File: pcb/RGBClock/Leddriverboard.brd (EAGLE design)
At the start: 68 x 41 mm, 37 parts, among them U1 LP3878MR-ADJ, U2 P82B96DR, U3 PCA9685PW, U4 ZXLD1362ET5TA, U5 ZXLD1362ET5TA, U6 ZXLD1362ET5TA, X1 43045-0400, X2 43045-0600

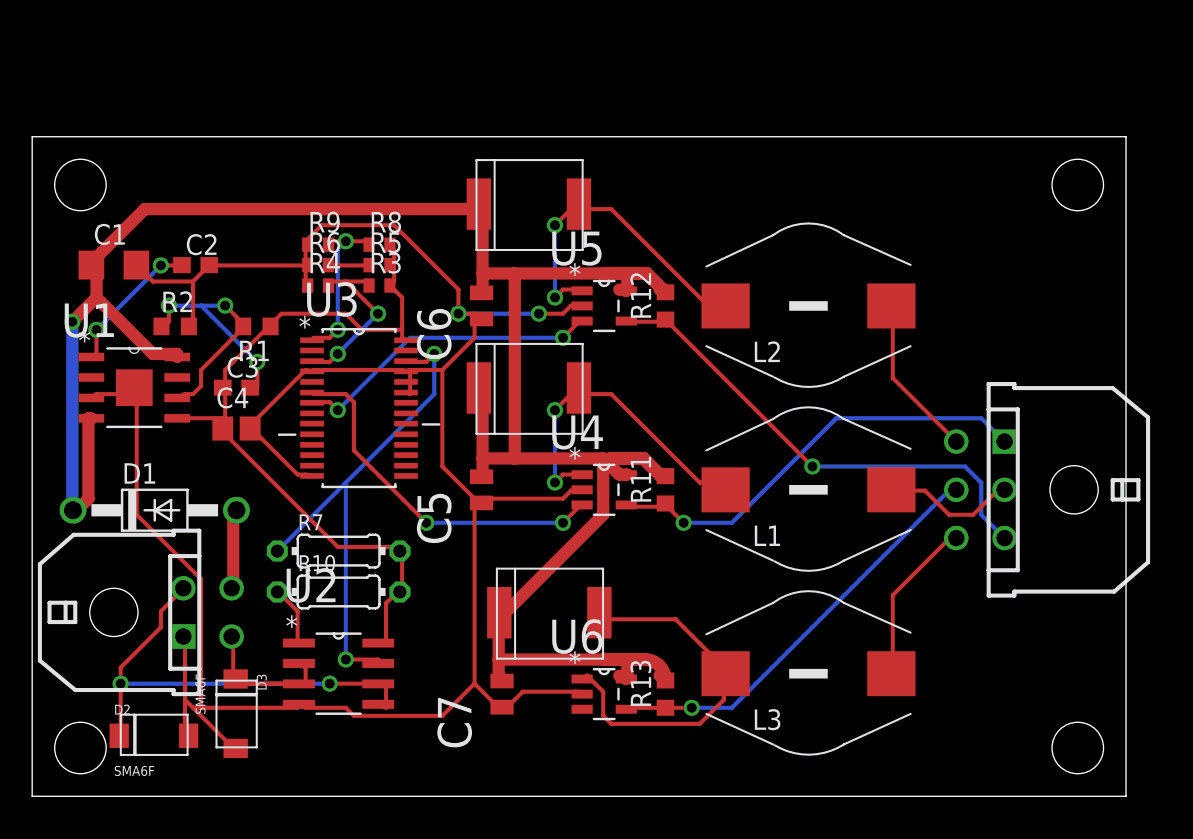
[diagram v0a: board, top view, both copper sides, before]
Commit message: Beta version master pcb (not complete routed !)
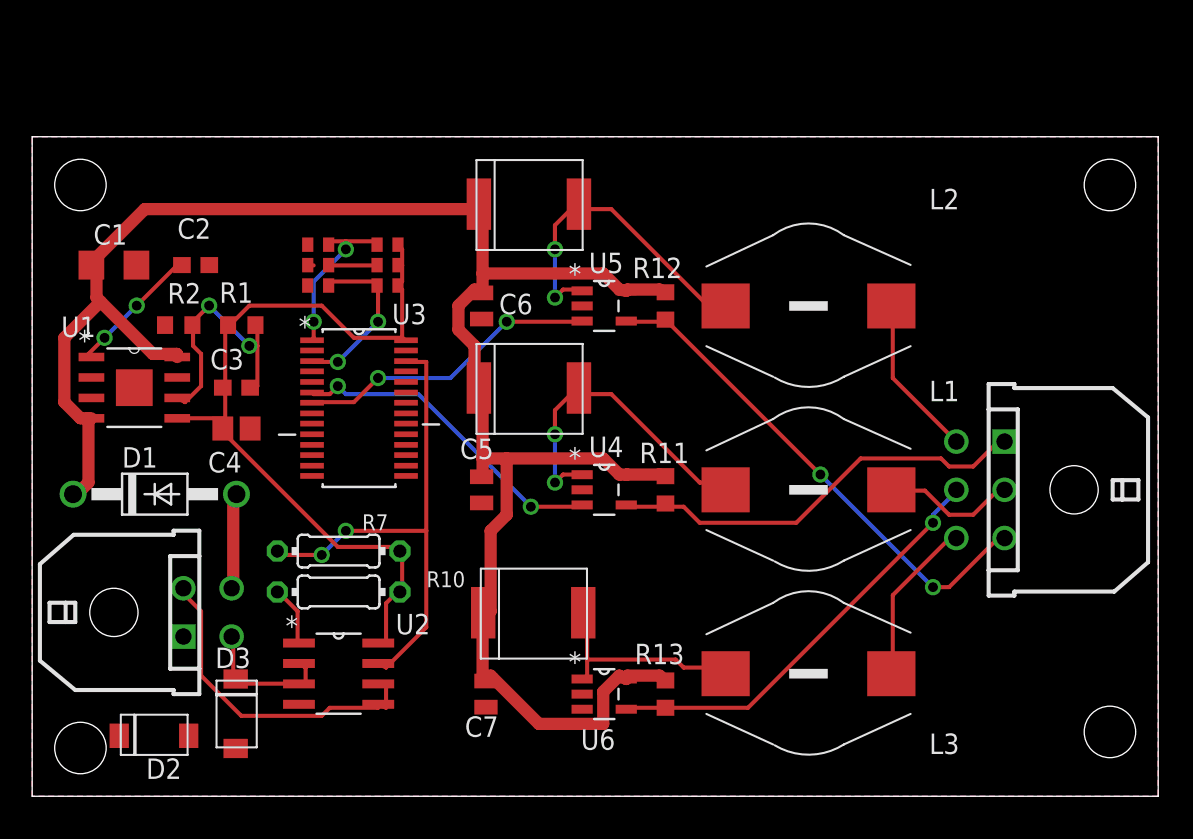
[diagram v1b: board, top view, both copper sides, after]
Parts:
- moved C7 1.00 mm to (28.2, 6.35)
- moved D1 1.00 mm to (7.62, 18.8)
- moved D6 1.00 mm to (29.5, 11.4)
- moved R1 0.94 mm to (13.0, 29.3), turned to 0 degrees
- moved R3 0.50 mm to (22.1, 31.8)
- moved R5 0.50 mm to (22.1, 33.0)
- moved R8 0.50 mm to (22.1, 34.3)
- moved R2 0.23 mm to (9.11, 29.3), turned to 180 degrees
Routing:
- net GND: track 153.7 -> 0.37 mm, vias 2 -> 0
- net VCC: track 135.1 -> 121.6 mm, vias 1 -> 0
- net N$19: track 22.9 -> 13.5 mm
- net N$22: track 29.3 -> 20.8 mm, vias 2 -> 0
- net N$24: track 20.2 -> 15.9 mm, vias 3 -> 2
- net N$8: track 22.3 -> 20.2 mm
- net +5V: track 48.1 -> 50.0 mm
- net N$4: track 30.3 -> 31.7 mm, vias 1 -> 2
- net N$25: track 4.97 -> 5.97 mm
- net N$1: track 27.4 -> 26.6 mm, vias 1 -> 0
- net N$42: track 2.64 -> 3.14 mm
- added copper zone on layer 1, net GND
- added copper zone on layer 16, net GND
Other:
- board size 68 x 41 mm -> 70 x 41 mm

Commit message: Just before freerouter
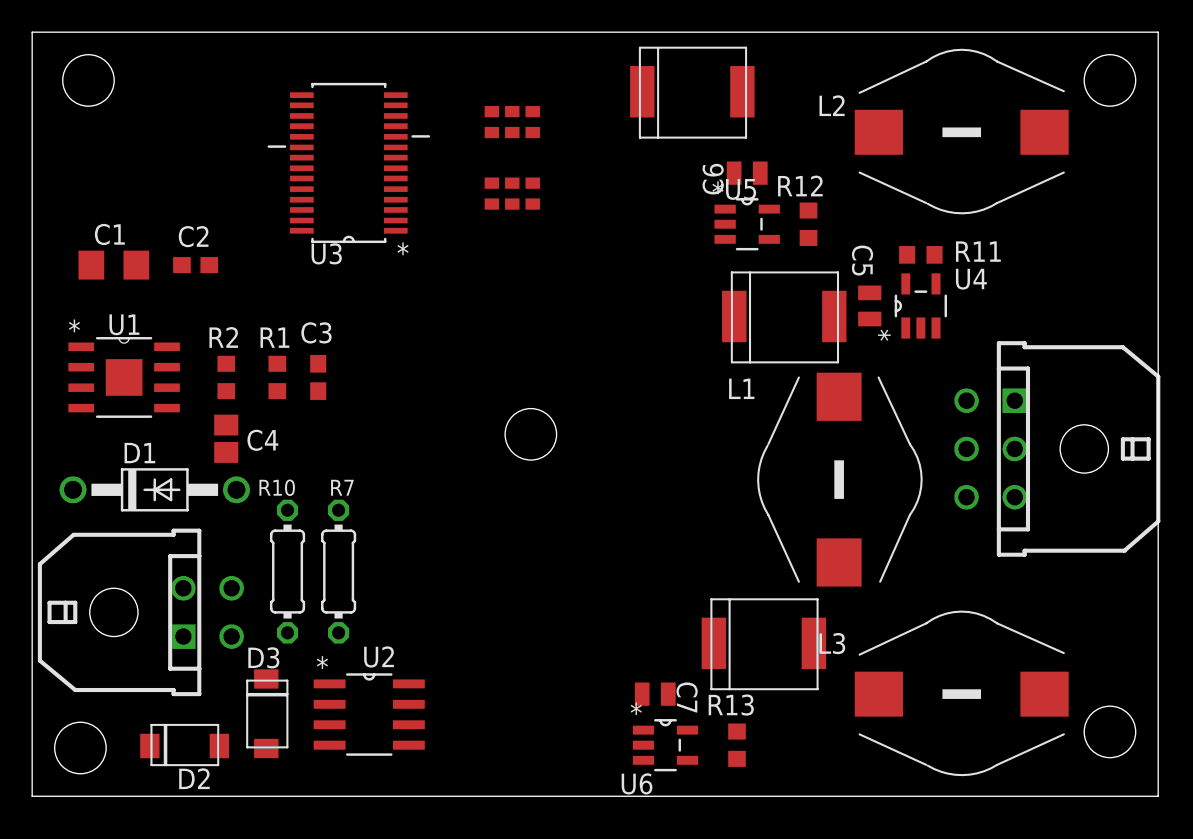
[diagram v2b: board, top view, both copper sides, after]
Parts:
- moved C5 26.7 mm to (52.1, 30.5)
- moved U4 22.8 mm to (55.2, 30.5), turned to 90 degrees
- moved R11 21.6 mm to (55.2, 33.7), turned to 180 degrees
- moved C6 18.5 mm to (44.5, 38.7), turned to 0 degrees
- moved D4 16.5 mm to (45.1, 29.8)
- moved R9 15.4 mm to (31.1, 41.9), turned to 270 degrees
- moved U3 15.3 mm to (19.7, 39.4), turned to 180 degrees
- moved R6 15.0 mm to (29.8, 41.9), turned to 270 degrees
- moved R4 14.8 mm to (28.6, 41.9), turned to 270 degrees
- moved D6 14.5 mm to (43.8, 9.53)
- moved L2 14.4 mm to (57.8, 41.3)
- moved D5 12.3 mm to (39.4, 43.8)
- moved C7 10.5 mm to (38.7, 6.35), turned to 0 degrees
- moved R12 10.2 mm to (48.3, 35.6)
- moved U5 10.2 mm to (44.5, 35.6)
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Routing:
- net VCC: track 121.6 -> 0.00 mm
- net +5V: track 50.0 -> 0.00 mm
- net SCL: track 31.8 -> 0.00 mm, vias 2 -> 0
- net N$4: track 31.7 -> 0.00 mm, vias 2 -> 0
- net N$1: track 26.6 -> 0.00 mm
- net N$16: track 26.6 -> 0.00 mm, vias 1 -> 0
- net N$22: track 20.8 -> 0.00 mm
- net N$10: track 20.6 -> 0.00 mm, vias 2 -> 0
- net N$9: track 20.3 -> 0.00 mm, vias 2 -> 0
- net N$8: track 20.2 -> 0.00 mm, vias 2 -> 0
- net N$2: track 18.9 -> 0.00 mm, vias 2 -> 0
- net N$24: track 15.9 -> 0.00 mm, vias 2 -> 0
- net N$19: track 13.5 -> 0.00 mm
- net N$43: track 10.9 -> 0.00 mm, vias 2 -> 0
- net N$41: track 10.5 -> 0.00 mm, vias 2 -> 0
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- removed copper zone on layer 1, net GND
- removed copper zone on layer 16, net GND
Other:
- board size 70 x 41 mm -> 70 x 47.5 mm
